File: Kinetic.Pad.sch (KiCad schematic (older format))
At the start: 20 parts, among them SW1 Rotary_Encoder_Switch, U1 ProMicro

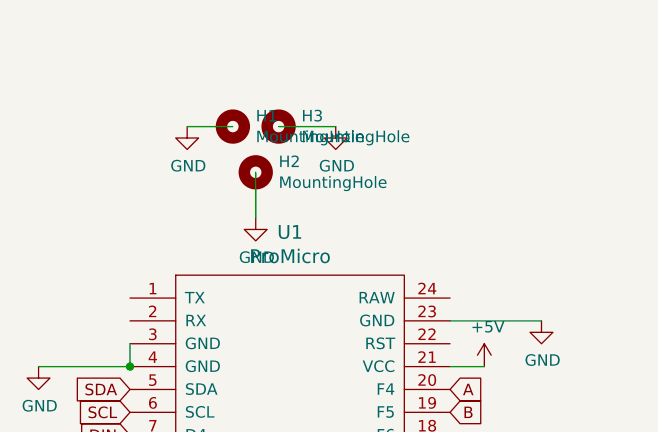
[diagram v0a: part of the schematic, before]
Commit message: Nothing Important
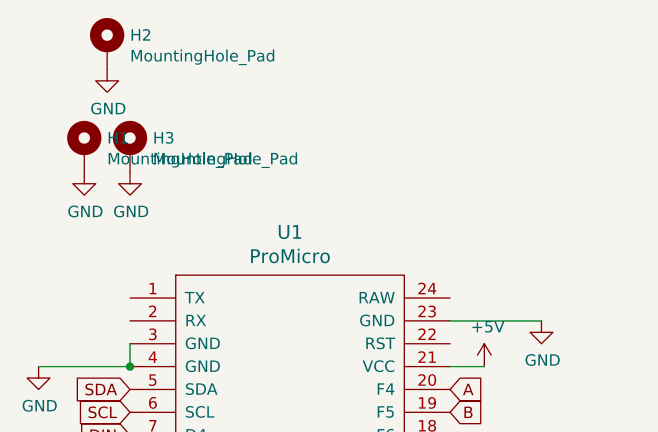
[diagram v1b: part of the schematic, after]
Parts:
- removed H1, H2, H3: MountingHole, MountingHole:MountingHole_2mm, symbol Mechanical:MountingHole
- added H1, H2, H3: MountingHole_Pad, MountingHole:MountingHole_2.5mm_Pad, symbol Mechanical:MountingHole_Pad
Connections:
- wire segments 26 -> 23
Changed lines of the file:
@@
 	4000 3900 4550 3900
 $Comp
-L Mechanical:MountingHole H1
-U 1 1 61AF6BAE
-P 2350 950
-F 0 "H1" H 2450 996 50  0000 L CNN
-F 1 "MountingHole" H 2450 905 50  0000 L CNN
-F 2 "MountingHole:MountingHole_2mm" H 2350 950 50  0001 C CNN
-F 3 "~" H 2350 950 50  0001 C CNN
-	1    2350 950
+L Mechanical:MountingHole_Pad H1
+U 1 1 61A9C773
+P 1700 1050
+F 0 "H1" H 1800 1099 50  0000 L CNN
+F 1 "MountingHole_Pad" H 1800 1008 50  0000 L CNN
+F 2 "MountingHole:MountingHole_2.5mm_Pad" H 1700 1050 50  0001 C CNN
+F 3 "~" H 1700 1050 50  0001 C CNN
+	1    1700 1050
 	1    0    0    -1
 $EndComp
 $Comp
-L Mechanical:MountingHole H3
-U 1 1 61AF77EB
-P 2550 950
-F 0 "H3" H 2650 996 50  0000 L CNN
-F 1 "MountingHole" H 2650 905 50  0000 L CNN
-F 2 "MountingHole:MountingHole_2mm" H 2550 950 50  0001 C CNN
-F 3 "~" H 2550 950 50  0001 C CNN
-	1    2550 950
+L Mechanical:MountingHole_Pad H3
+U 1 1 61A9D1A0
+P 1900 1050
+F 0 "H3" H 2000 1099 50  0000 L CNN
+F 1 "MountingHole_Pad" H 2000 1008 50  0000 L CNN
+F 2 "MountingHole:MountingHole_2.5mm_Pad" H 1900 1050 50  0001 C CNN
+F 3 "~" H 1900 1050 50  0001 C CNN
+	1    1900 1050
 	1    0    0    -1
 $EndComp
 $Comp
-L Mechanical:MountingHole H2
-U 1 1 61AF7FA8
-P 2450 1150
-F 0 "H2" H 2550 1196 50  0000 L CNN
-F 1 "MountingHole" H 2550 1105 50  0000 L CNN
-F 2 "MountingHole:MountingHole_2mm" H 2450 1150 50  0001 C CNN
-F 3 "~" H 2450 1150 50  0001 C CNN
-	1    2450 1150
+L Mechanical:MountingHole_Pad H2
+U 1 1 61A9D90B
+P 1800 600
+F 0 "H2" H 1900 649 50  0000 L CNN
+F 1 "MountingHole_Pad" H 1900 558 50  0000 L CNN
+F 2 "MountingHole:MountingHole_2.5mm_Pad" H 1800 600 50  0001 C CNN
+F 3 "~" H 1800 600 50  0001 C CNN
+	1    1800 600
 	1    0    0    -1
 $EndComp
-Wire Wire Line
-	2550 950  2800 950
-Wire Wire Line
-	2450 1150 2450 1350
-Wire Wire Line
-	2350 950  2150 950
 $Comp
 L power:GND #PWR0110
-U 1 1 61A99687
-P 2800 950
-F 0 "#PWR0110" H 2800 700 50  0001 C CNN
-F 1 "GND" H 2805 777 50  0000 C CNN
-F 2 "" H 2800 950 50  0001 C CNN
-F 3 "" H 2800 950 50  0001 C CNN
-	1    2800 950
+U 1 1 61AA5B29
+P 1700 1150
+F 0 "#PWR0110" H 1700 900 50  0001 C CNN
+F 1 "GND" H 1705 977 50  0000 C CNN
+F 2 "" H 1700 1150 50  0001 C CNN
+F 3 "" H 1700 1150 50  0001 C CNN
+	1    1700 1150
 	1    0    0    -1
 $EndComp
 $Comp
 L power:GND #PWR0111
-U 1 1 61A99FC8
-P 2450 1350
-F 0 "#PWR0111" H 2450 1100 50  0001 C CNN
-F 1 "GND" H 2455 1177 50  0000 C CNN
-F 2 "" H 2450 1350 50  0001 C CNN
-F 3 "" H 2450 1350 50  0001 C CNN
-	1    2450 1350
+U 1 1 61AA6232
+P 1900 1150
+F 0 "#PWR0111" H 1900 900 50  0001 C CNN
+F 1 "GND" H 1905 977 50  0000 C CNN
+F 2 "" H 1900 1150 50  0001 C CNN
+F 3 "" H 1900 1150 50  0001 C CNN
+	1    1900 1150
 	1    0    0    -1
 $EndComp
 $Comp
 L power:GND #PWR0115
-U 1 1 61A9A984
-P 2150 950
-F 0 "#PWR0115" H 2150 700 50  0001 C CNN
-F 1 "GND" H 2155 777 50  0000 C CNN
-F 2 "" H 2150 950 50  0001 C CNN
-F 3 "" H 2150 950 50  0001 C CNN
-	1    2150 950
+U 1 1 61AA723D
+P 1800 700
+F 0 "#PWR0115" H 1800 450 50  0001 C CNN
+F 1 "GND" H 1805 527 50  0000 C CNN
+F 2 "" H 1800 700 50  0001 C CNN
+F 3 "" H 1800 700 50  0001 C CNN
+	1    1800 700
 	1    0    0    -1
 $EndComp
